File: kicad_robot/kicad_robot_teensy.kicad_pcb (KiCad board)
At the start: 2 copper layers, 23 parts, among them J1 Conn_01x04_Male, J2 Conn_01x04_Male, Q1 IRLML0030, U12->5 R-78E5.0-1.0

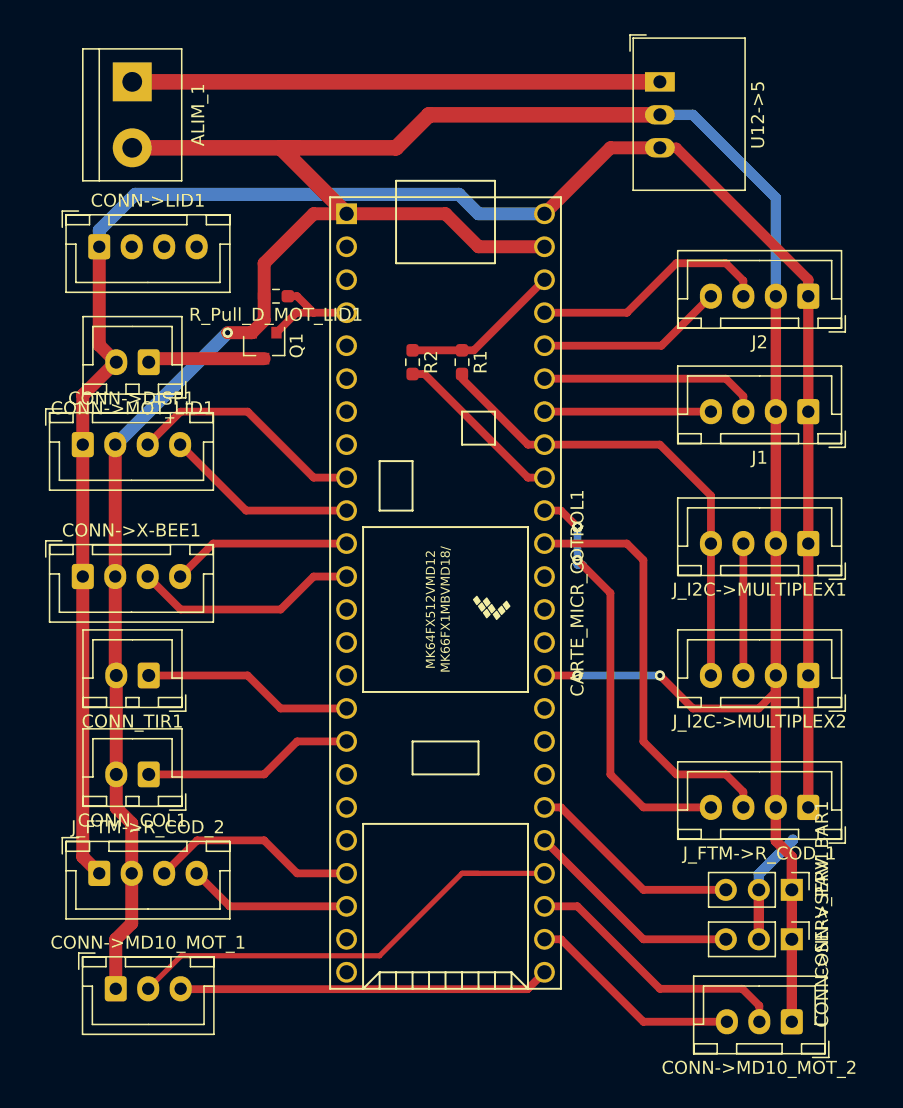
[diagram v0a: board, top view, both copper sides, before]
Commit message: Teensy V2.1: Carte presque prête
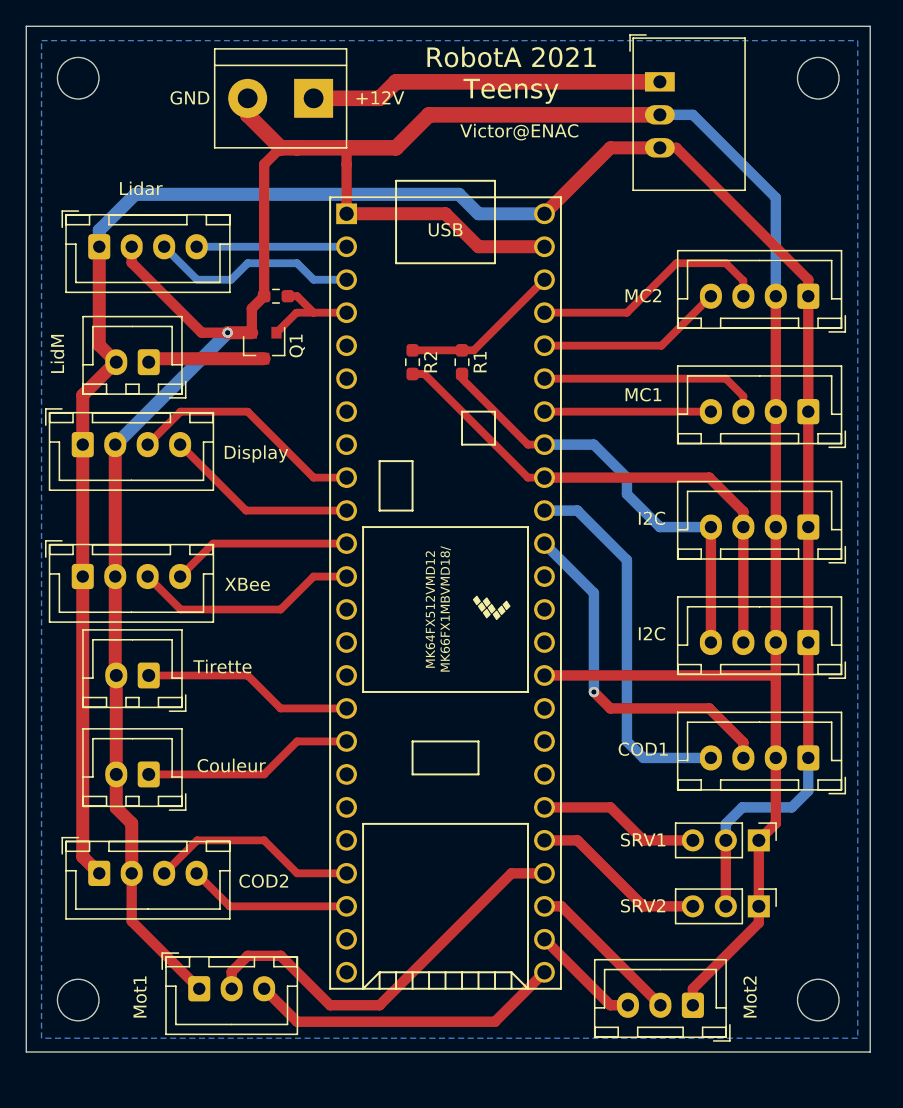
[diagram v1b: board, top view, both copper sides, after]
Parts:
- added REF**: MountingHole_3.2mm_M3, MountingHole:MountingHole_3.2mm_M3, F.Cu at (190.0, 152.0)
- added REF**: MountingHole_3.2mm_M3, MountingHole:MountingHole_3.2mm_M3, F.Cu at (133.0, 152.0)
- added REF**: MountingHole_3.2mm_M3, MountingHole:MountingHole_3.2mm_M3, F.Cu at (133.0, 81.0)
- added REF**: MountingHole_3.2mm_M3, MountingHole:MountingHole_3.2mm_M3, F.Cu at (190.0, 81.0)
- moved ALIM_1 14.0 mm to (151.1, 82.5), turned to 180 degrees
- moved CONN->MD10_MOT_2 7.73 mm to (180.3, 152.4)
- moved CONN->MD10_MOT_1 6.43 mm to (142.3, 151.1)
- moved CONN->SERV_BAR1 4.58 mm to (185.4, 139.7)
- moved J_FTM->R_COD_1 3.81 mm to (189.2, 133.3)
- moved CONN->SERV_PAV1 3.59 mm to (185.4, 144.8)
- moved J_I2C->MULTIPLEX2 2.54 mm to (189.2, 124.5)
- moved J_I2C->MULTIPLEX1 1.27 mm to (189.2, 115.6)
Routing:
- net I2C_SDAO: track 23.6 -> 39.9 mm
- net LID_TX: track 0.00 -> 16.2 mm
- net +12V: track 40.6 -> 27.2 mm
- net LID_RX: track 0.00 -> 11.5 mm
- net MOT_2_PWM: track 21.0 -> 12.1 mm
- net MOT_2_DIR: track 16.7 -> 8.53 mm
- net R_COD_1_phA: track 32.6 -> 27.3 mm, vias 0 -> 1
- net MOT_1_DIR: track 28.6 -> 24.2 mm
- net BAR_SERV: track 16.6 -> 12.5 mm
- net R_COD_1_phB: track 32.8 -> 28.9 mm, vias 3 -> 0
- net MOT_1_PWM: track 35.5 -> 31.7 mm
- net +5V: track 163.8 -> 167.5 mm
- net PAV_SERV: track 17.1 -> 13.5 mm
- net I2C_SCLO: track 36.8 -> 33.5 mm
- net GND: track 233.3 -> 235.4 mm, vias 4 -> 2
- added copper zone on B.Cu, net GND
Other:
- board outline added: 65 x 79 mm
- board text added: "+12V"
- board text added: "COD1"
- board text added: "COD2"
- board text added: "Couleur"
- board text added: "Display"
- board text added: "GND"
- board text added: "I2C"
- board text added: "LidM"
- board text added: "Lidar"
- board text added: "MC1"
- board text added: "MC2"
- board text added: "Mot1"
- board text added: "Mot2"
- board text added: "RobotA 2021 Teensy"
- board text added: "SRV1"
- board text added: "SRV2"
- board text added: "Tirette"
- board text added: "USB"
- board text added: "Victor@ENAC"
- board text added: "XBee"
